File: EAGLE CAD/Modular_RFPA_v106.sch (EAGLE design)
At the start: 197 parts, among them IC301 74AHC1G14DBV, IC302 LM324D, J401 FUSE_2P, J402 KK_PCFAN, Q101 IRF520N, Q102 IRF630, Q201 IRF630, Q202 IRF630, Q301 BSS123, T101 HP4_TRAFO, T102 HP4_TRAFO, X402 HEATSINK_OMNI_DUAL30-75-D

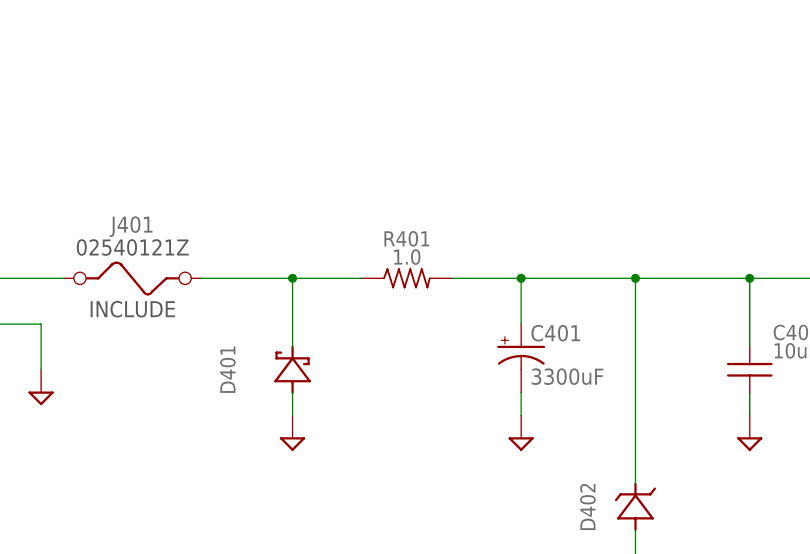
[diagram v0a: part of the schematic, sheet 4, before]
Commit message: .
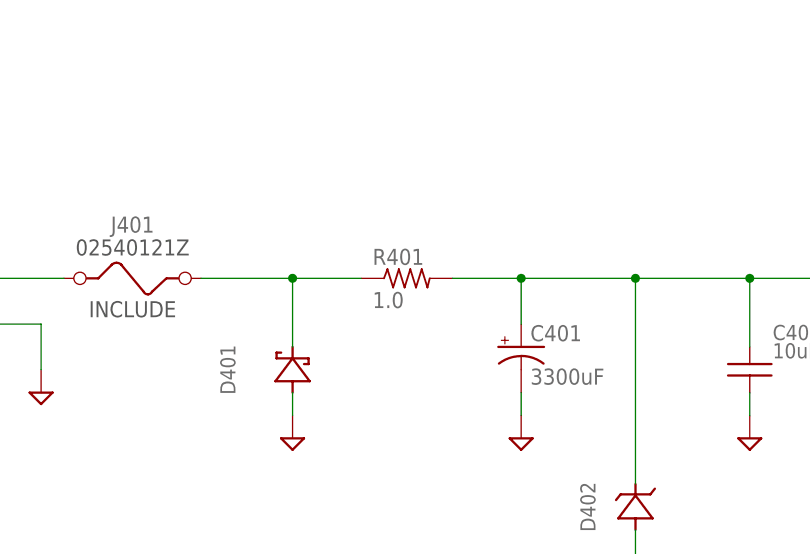
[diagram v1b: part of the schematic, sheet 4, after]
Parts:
- R401: device MDT_R:R90R-1.0K-1%-1206-0.25WR1206 -> resistor:R-US_0817/7V
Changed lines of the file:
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@@
 <grid distance="0.1" unitdist="inch" unit="inch" style="lines" multiple="1" display="no" altdistance="0.01" altunitdist="inch" altunit="inch"/>
 <layers>
-<layer number="1" name="Top" color="4" fill="1" visible="yes" active="no"/>
-<layer number="2" name="Route2" color="1" fill="3" visible="yes" active="no"/>
-<layer number="3" name="Route3" color="4" fill="3" visible="yes" active="no"/>
-<layer number="4" name="Route4" color="1" fill="4" visible="yes" active="no"/>
-<layer number="5" name="Route5" color="4" fill="4" visible="yes" active="no"/>
-<layer number="6" name="Route6" color="1" fill="8" visible="yes" active="no"/>
-<layer number="7" name="Route7" color="4" fill="8" visible="yes" active="no"/>
-<layer number="8" name="Route8" color="1" fill="2" visible="yes" active="no"/>
-<layer number="9" name="Route9" color="4" fill="2" visible="yes" active="no"/>
-<layer number="10" name="Route10" color="1" fill="7" visible="yes" active="no"/>
-<layer number="11" name="Route11" color="4" fill="7" visible="yes" active="no"/>
-<layer number="12" name="Route12" color="1" fill="5" visible="yes" active="no"/>
-<layer number="13" name="Route13" color="4" fill="5" visible="yes" active="no"/>
-<layer number="14" name="Route14" color="1" fill="6" visible="yes" active="no"/>
-<layer number="15" name="Route15" color="4" fill="6" visible="yes" active="no"/>
-<layer number="16" name="Bottom" color="1" fill="1" visible="yes" active="no"/>
-<layer number="17" name="Pads" color="2" fill="1" visible="yes" active="no"/>
-<layer number="18" name="Vias" color="2" fill="1" visible="yes" active="no"/>
-<layer number="19" name="Unrouted" color="6" fill="1" visible="yes" active="no"/>
-<layer number="20" name="Dimension" color="15" fill="1" visible="yes" active="no"/>
-<layer number="21" name="tPlace" color="7" fill="1" visible="yes" active="no"/>
-<layer number="22" name="bPlace" color="7" fill="1" visible="yes" active="no"/>
-<layer number="23" name="tOrigins" color="15" fill="1" visible="yes" active="no"/>
-<layer number="24" name="bOrigins" color="15" fill="1" visible="yes" active="no"/>
-<layer number="25" name="tNames" color="7" fill="1" visible="yes" active="no"/>
-<layer number="26" name="bNames" color="7" fill="1" visible="yes" active="no"/>
-<layer number="27" name="tValues" color="7" fill="1" visible="yes" active="no"/>
-<layer number="28" name="bValues" color="7" fill="1" visible="yes" active="no"/>
+<layer number="1" name="Top" color="4" fill="1" visible="no" active="no"/>
+<layer number="2" name="Route2" color="1" fill="3" visible="no" active="no"/>
+<layer number="3" name="Route3" color="4" fill="3" visible="no" active="no"/>
+<layer number="4" name="Route4" color="1" fill="4" visible="no" active="no"/>
+<layer number="5" name="Route5" color="4" fill="4" visible="no" active="no"/>
+<layer number="6" name="Route6" color="1" fill="8" visible="no" active="no"/>
+<layer number="7" name="Route7" color="4" fill="8" visible="no" active="no"/>
+<layer number="8" name="Route8" color="1" fill="2" visible="no" active="no"/>
+<layer number="9" name="Route9" color="4" fill="2" visible="no" active="no"/>
+<layer number="10" name="Route10" color="1" fill="7" visible="no" active="no"/>
+<layer number="11" name="Route11" color="4" fill="7" visible="no" active="no"/>
+<layer number="12" name="Route12" color="1" fill="5" visible="no" active="no"/>
+<layer number="13" name="Route13" color="4" fill="5" visible="no" active="no"/>
+<layer number="14" name="Route14" color="1" fill="6" visible="no" active="no"/>
+<layer number="15" name="Route15" color="4" fill="6" visible="no" active="no"/>
+<layer number="16" name="Bottom" color="1" fill="1" visible="no" active="no"/>
+<layer number="17" name="Pads" color="2" fill="1" visible="no" active="no"/>
+<layer number="18" name="Vias" color="2" fill="1" visible="no" active="no"/>
+<layer number="19" name="Unrouted" color="6" fill="1" visible="no" active="no"/>
+<layer number="20" name="Dimension" color="15" fill="1" visible="no" active="no"/>
+<layer number="21" name="tPlace" color="7" fill="1" visible="no" active="no"/>
+<layer number="22" name="bPlace" color="7" fill="1" visible="no" active="no"/>
+<layer number="23" name="tOrigins" color="15" fill="1" visible="no" active="no"/>
+<layer number="24" name="bOrigins" color="15" fill="1" visible="no" active="no"/>
+<layer number="25" name="tNames" color="7" fill="1" visible="no" active="no"/>
+<layer number="26" name="bNames" color="7" fill="1" visible="no" active="no"/>
+<layer number="27" name="tValues" color="7" fill="1" visible="no" active="no"/>
+<layer number="28" name="bValues" color="7" fill="1" visible="no" active="no"/>
 <layer number="29" name="tStop" color="7" fill="3" visible="no" active="no"/>
 <layer number="30" name="bStop" color="7" fill="6" visible="no" active="no"/>
@@
 <layer number="35" name="tGlue" color="7" fill="4" visible="no" active="no"/>
 <layer number="36" name="bGlue" color="7" fill="5" visible="no" active="no"/>
-<layer number="37" name="tTest" color="7" fill="1" visible="yes" active="no"/>
-<layer number="38" name="bTest" color="7" fill="1" visible="yes" active="no"/>
+<layer number="37" name="tTest" color="7" fill="1" visible="no" active="no"/>
+<layer number="38" name="bTest" color="7" fill="1" visible="no" active="no"/>
 <layer number="39" name="tKeepout" color="4" fill="11" visible="no" active="no"/>
 <layer number="40" name="bKeepout" color="1" fill="11" visible="no" active="no"/>
@@
 <layer number="44" name="Drills" color="7" fill="1" visible="no" active="no"/>
 <layer number="45" name="Holes" color="7" fill="1" visible="no" active="no"/>
-<layer number="46" name="Milling" color="3" fill="1" visible="yes" active="no"/>
-<layer number="47" name="Measures" color="7" fill="1" visible="yes" active="no"/>
-<layer number="48" name="Document" color="7" fill="1" visible="yes" active="no"/>
-<layer number="49" name="Reference" color="7" fill="1" visible="yes" active="no"/>
-<layer number="50" name="dxf" color="7" fill="1" visible="yes" active="no"/>
-<layer number="51" name="tDocu" color="7" fill="1" visible="yes" active="no"/>
-<layer number="52" name="bDocu" color="7" fill="1" visible="yes" active="no"/>
-<layer number="56" name="wert" color="7" fill="1" visible="yes" active="no"/>
+<layer number="46" name="Milling" color="3" fill="1" visible="no" active="no"/>
+<layer number="47" name="Measures" color="7" fill="1" visible="no" active="no"/>
+<layer number="48" name="Document" color="7" fill="1" visible="no" active="no"/>
+<layer number="49" name="Reference" color="7" fill="1" visible="no" active="no"/>
+<layer number="50" name="dxf" color="7" fill="1" visible="no" active="no"/>
+<layer number="51" name="tDocu" color="7" fill="1" visible="no" active="no"/>
+<layer number="52" name="bDocu" color="7" fill="1" visible="no" active="no"/>
+<layer number="56" name="wert" color="7" fill="1" visible="no" active="no"/>
 <layer number="90" name="Modules" color="5" fill="1" visible="yes" active="yes"/>
 <layer number="91" name="Nets" color="2" fill="1" visible="yes" active="yes"/>
@@
 </attributes>
 <variantdefs>
-<variantdef name="IRF520N_20W" current="yes"/>
+<variantdef name="IRF520N_20W"/>
 <variantdef name="IRF630_200W"/>
 </variantdefs>
@@
 <part name="D401" library="MDT_Diode" deviceset="D-SCHOTTKY" device="SMC" technology="SK810L-TP" value="D-SCHOTTKYSK810L-TPSMC"/>
 <part name="SUPPLY402" library="supply2" deviceset="GND" device=""/>
-<part name="R401" library="MDT_R" deviceset="R90" device="R1206" technology="R-1.0K-1%-1206-0.25W" value="1.0"/>
+<part name="R401" library="resistor" deviceset="R-US_" device="0817/7V" value="1.0"/>
 <part name="C401" library="rcl" deviceset="CPOL-US" device="E10-25" value="3300uF"/>
 <part name="SUPPLY403" library="supply2" deviceset="GND" device=""/>
